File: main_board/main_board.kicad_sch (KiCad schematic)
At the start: 6 parts, among them J1 Conn_01x04_Socket, J2 Conn_01x04, J3 Conn_02x03_Odd_Even, J4 Conn_02x01, J5 Conn_02x02_Odd_Even, U1 Pico

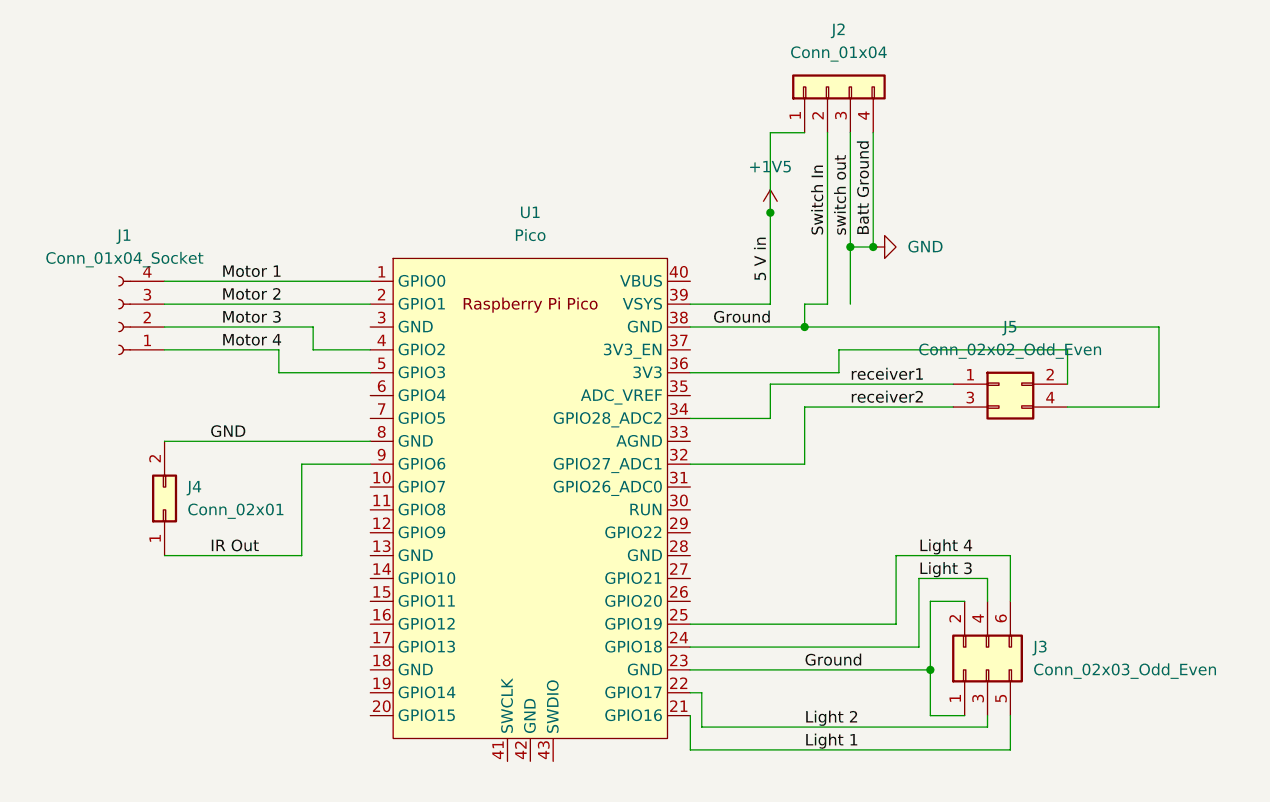
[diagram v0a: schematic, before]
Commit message: first commit
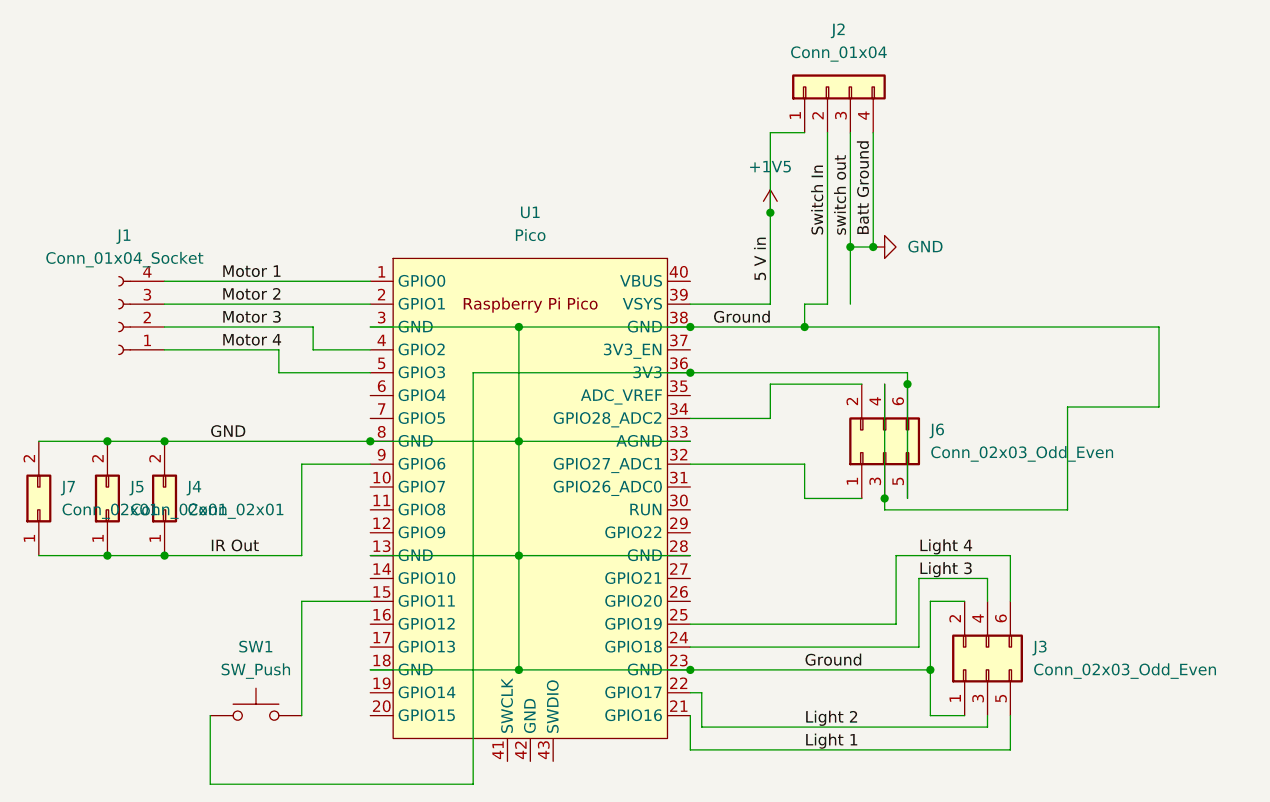
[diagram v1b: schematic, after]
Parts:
- removed J5: Conn_02x02_Odd_Even, Connector_PinHeader_2.54mm:PinHeader_2x02_P2.54mm_Vertical, symbol Connector_Generic:Conn_02x02_Odd_Even
- added J5, J7: Conn_02x01, Connector_PinHeader_2.54mm:PinHeader_2x01_P2.54mm_Vertical, symbol Connector_Generic:Conn_02x01
- added J6: Conn_02x03_Odd_Even, Connector_PinHeader_2.54mm:PinHeader_2x03_P2.54mm_Vertical, symbol Connector_Generic:Conn_02x03_Odd_Even
- added SW1: SW_Push, Button_Switch_SMD:SW_Push_1P1T_NO_CK_PTS125Sx43PSMTR, symbol Switch:SW_Push
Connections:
- net Ground is gone; now on net GND: J2.2 (Pin_2), J3.1 (Pin_1), J3.2 (Pin_2), U1.23 (GND), U1.38 (GND)
- net GND: now also U1.13 (GND), U1.18 (GND), U1.28 (GND), U1.3 (GND), U1.33 (AGND), J5.2 (Pin_2), J6.3 (Pin_3), J6.4 (Pin_4), J7.2 (Pin_2)
- net IR Out: now also J5.1 (Pin_1), J7.1 (Pin_1)
- net at U1.15 (GPIO11): now also SW1.2
- net at U1.36 (3V3): now also J6.5 (Pin_5), J6.6 (Pin_6), SW1.1
- net receiver1: no longer names the net of U1.34 (GPIO28_ADC2)
- net receiver1: now also J6.2 (Pin_2)
- net receiver2: no longer names the net of U1.32 (GPIO27_ADC1)
- net receiver2: now also J6.1 (Pin_1)
